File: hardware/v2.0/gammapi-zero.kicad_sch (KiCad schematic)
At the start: 25 parts, among them J1 Conn_02x20_Counter_Clockwise, SW1 SW_Push, SW2 SW_Push, U1 ECP5U-25F-CABGA256, Y1 SG-8018CG 50.000000MHz

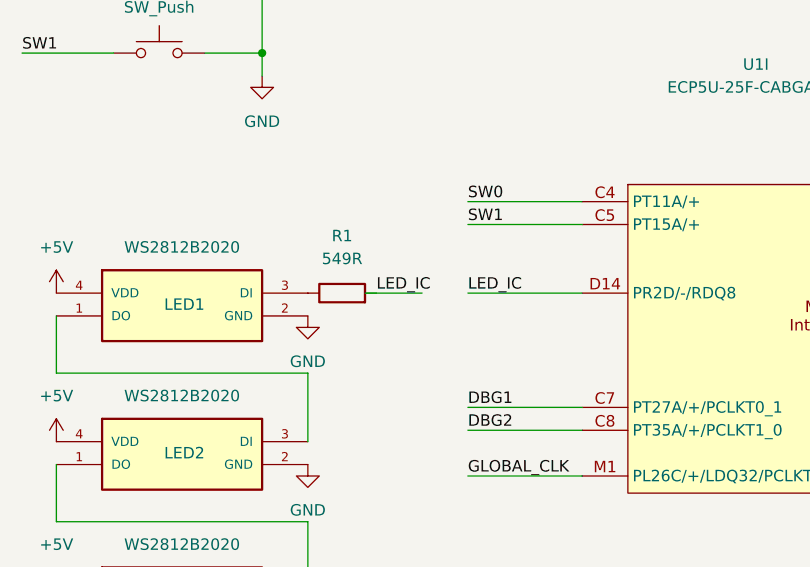
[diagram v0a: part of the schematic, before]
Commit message: Capacitor update
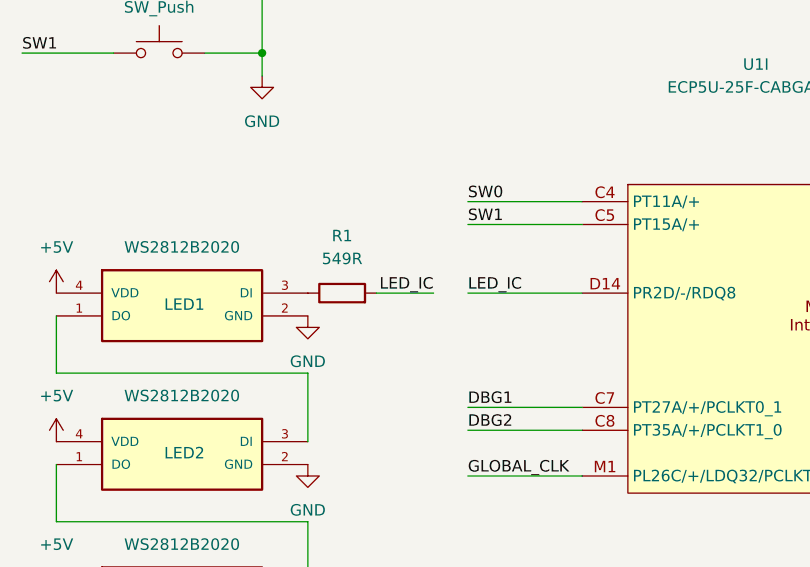
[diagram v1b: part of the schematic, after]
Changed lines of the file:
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@@
 	(wire
 		(pts
-			(xy 59.69 116.84) (xy 66.04 116.84)
+			(xy 60.96 116.84) (xy 67.31 116.84)
 		)
 		(stroke
@@
 	)
 	(label "LED_IC"
-		(at 60.96 116.84 0)
-		(effects
-			(font
-				(size 1.27 1.27)
-			)
-			(justify left bottom)
-		)
-	)
+		(at 67.31 116.84 180)
+		(effects
+			(font
+				(size 1.27 1.27)
+			)
+			(justify right bottom)
+		)
+	)
